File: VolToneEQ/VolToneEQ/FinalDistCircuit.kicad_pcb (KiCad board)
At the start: 4 copper layers, 96.8 x 83.6 mm, 94 parts, among them Q1 ZTX951, Q2 ZTX951, U1 TL072, U2 TL072, U3 TL072, U4 TL072

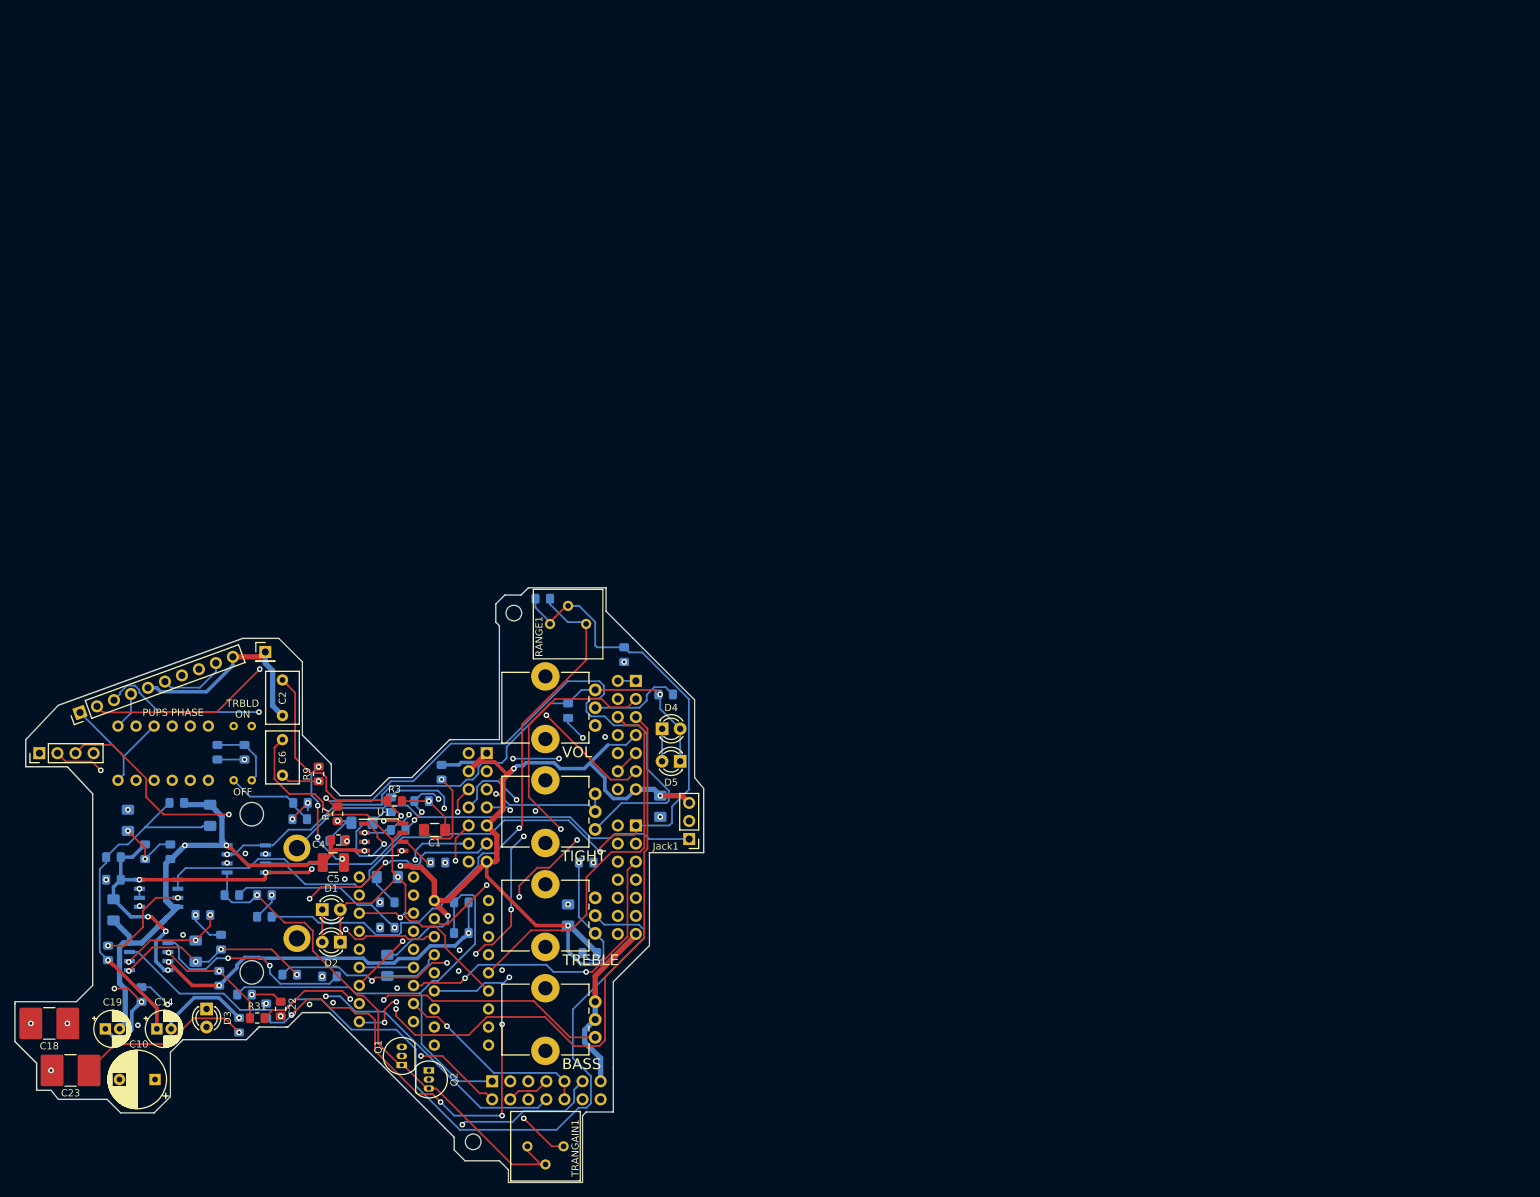
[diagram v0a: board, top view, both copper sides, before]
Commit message: fucked it up. gotta redo
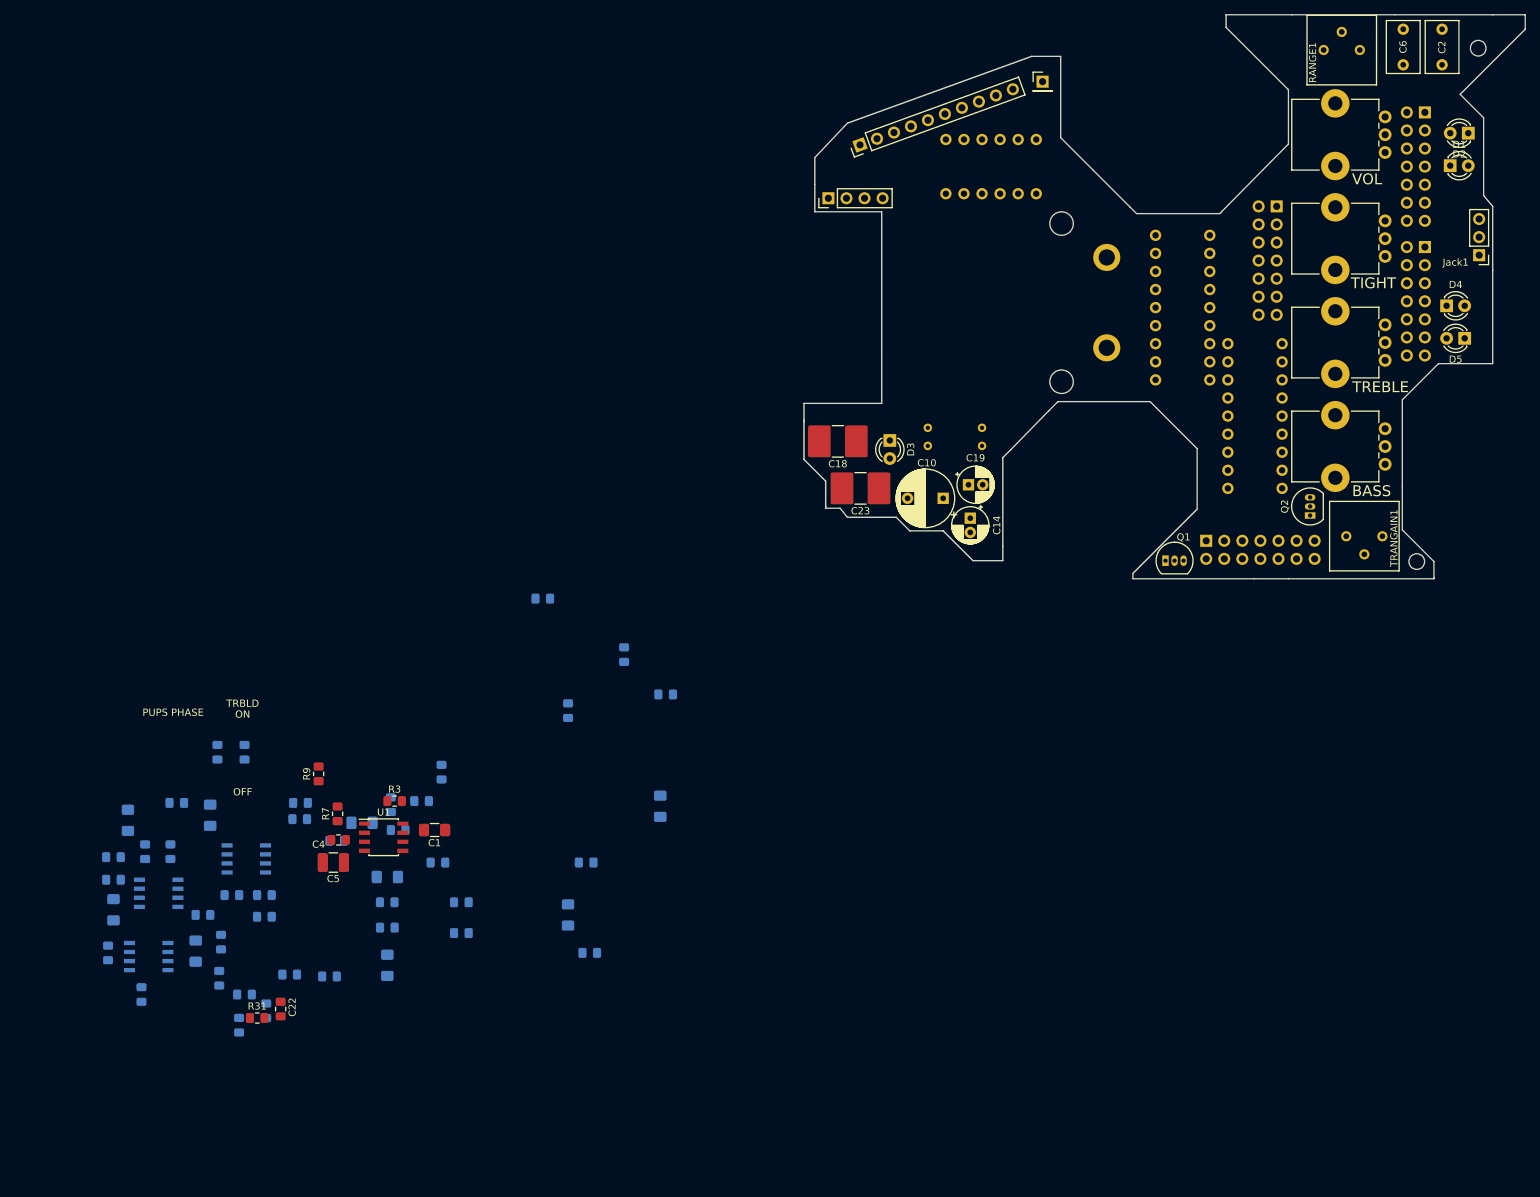
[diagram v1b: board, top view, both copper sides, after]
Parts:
- moved D2 195.0 mm to (248.4, 41.8)
- moved D1 189.9 mm to (245.9, 46.4)
- moved C2 186.8 mm to (244.7, 27.2)
- moved C6 186.5 mm to (239.3, 27.2)
- moved REF** 157.0 mm to (249.8, 29.8)
- moved REF** 155.7 mm to (241.2, 102.0)
- moved NeckTonePot1 149.4 mm to (242.3, 38.9)
- moved Q2 146.3 mm to (226.2, 95.5), turned to 90 degrees
- moved 6pdt1 143.7 mm to (207.0, 84.1)
- moved TRANGAIN1 143.5 mm to (231.3, 98.4)
- moved C19 143.4 mm to (178.2, 91.2)
- moved 4pdt1 142.6 mm to (200.4, 47.8)
- moved 9V1 140.8 mm to (146.8, 71.9)
- moved Jack1 138.0 mm to (249.9, 58.9)
- moved C23 137.9 mm to (163.0, 91.7)
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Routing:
- net BRGRN2: track 388.4 -> 0.00 mm, vias 11 -> 0
- net NBLACK: track 127.9 -> 0.00 mm
- net PRESIN: track 119.6 -> 0.00 mm, vias 1 -> 0
- net Net-(TREBLE1-Pad2): track 118.3 -> 0.00 mm
- net NVOUTTRAD: track 108.3 -> 0.00 mm
- net BRBLACK: track 100.4 -> 0.00 mm, vias 2 -> 0
- net ODMIDIN: track 99.8 -> 0.00 mm, vias 4 -> 0
- net BRRED2: track 99.2 -> 0.00 mm, vias 3 -> 0
- net Vref2: track 99.1 -> 0.00 mm, vias 3 -> 0
- net NOUT: track 98.6 -> 0.00 mm, vias 3 -> 0
- net NGRN2: track 97.5 -> 0.00 mm, vias 2 -> 0
- net BRWHT: track 93.9 -> 0.00 mm, vias 2 -> 0
- net Net-(C10-Pad1): track 88.9 -> 0.00 mm, vias 8 -> 0
- net BTONEIN: track 88.6 -> 0.00 mm, vias 1 -> 0
- net Net-(BASS1-Pad3): track 86.9 -> 0.00 mm, vias 3 -> 0
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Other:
- board size 96.8 x 83.6 mm -> 101.3 x 79.2 mm
